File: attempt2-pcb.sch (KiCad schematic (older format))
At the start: 15 parts, among them J1 Conn_01x04, SW1 SW_Push, U1 ATmega32U4-AU, Y1 16MHz

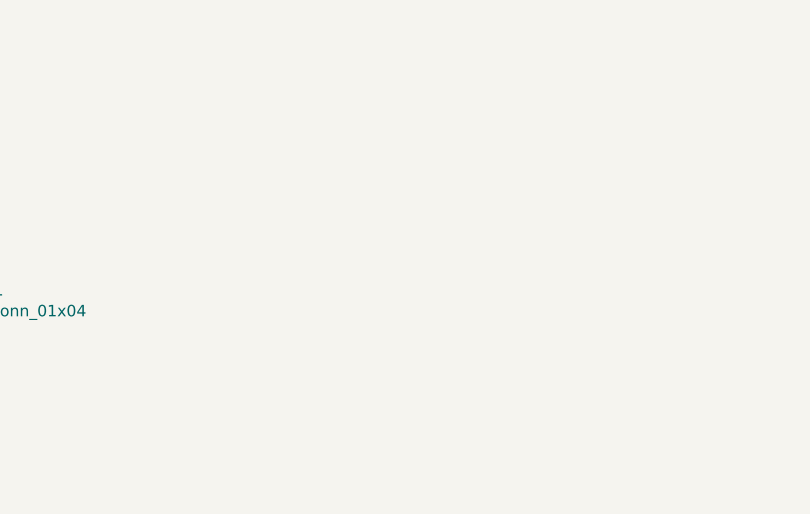
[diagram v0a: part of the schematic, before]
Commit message: PCB prep actually finished
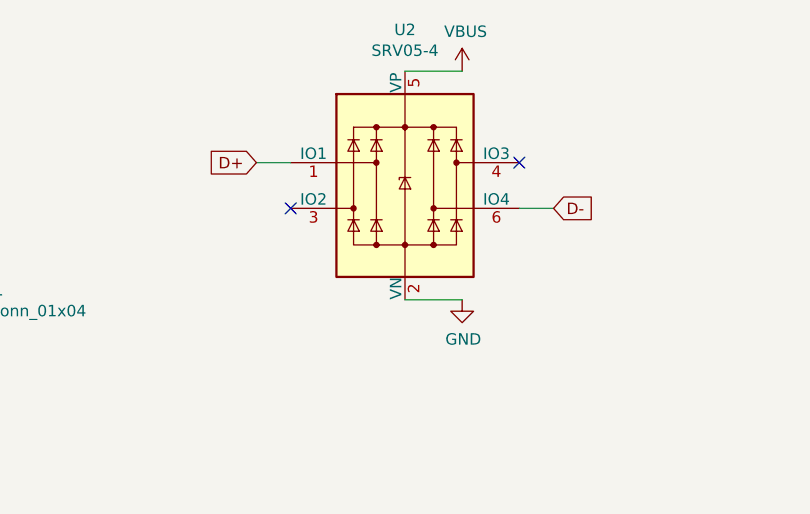
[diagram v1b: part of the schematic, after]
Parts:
- added U2: SRV05-4, Package_TO_SOT_SMD:SOT-23-6, symbol Power_Protection:SRV05-4
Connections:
- net D+: now also U2.1 (IO1)
- net D-: now also U2.6 (IO4)
- net GND: now also U2.2 (VN)
- net VBUS: now also U2.5 (VP)
- no-connect marks 0 -> 2
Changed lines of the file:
@@
 Text GLabel 1050 2350 0    50   Input ~ 0
 D+
+$Comp
+L Power_Protection:SRV05-4 U2
+U 1 1 6234A89E
+P 3300 1800
+F 0 "U2" H 3300 2481 50  0000 C CNN
+F 1 "SRV05-4" H 3300 2390 50  0000 C CNN
+F 2 "Package_TO_SOT_SMD:SOT-23-6" H 4000 1350 50  0001 C CNN
+F 3 "http://www.onsemi.com/pub/Collateral/SRV05-4-D.PDF" H 3300 1800 50  0001 C CNN
+	1    3300 1800
+	1    0    0    -1
+$EndComp
+NoConn ~ 3800 1700
+NoConn ~ 2800 1900
+Wire Wire Line
+	2800 1700 2650 1700
+Wire Wire Line
+	3800 1900 3950 1900
+Text GLabel 2650 1700 0    50   Input ~ 0
+D+
+Text GLabel 3950 1900 2    50   Input ~ 0
+D-
+Wire Wire Line
+	3300 2300 3550 2300
+$Comp
+L power:GND #PWR0113
+U 1 1 623564EB
+P 3550 2300
+F 0 "#PWR0113" H 3550 2050 50  0001 C CNN
+F 1 "GND" H 3555 2127 50  0000 C CNN
+F 2 "" H 3550 2300 50  0001 C CNN
+F 3 "" H 3550 2300 50  0001 C CNN
+	1    3550 2300
+	1    0    0    -1
+$EndComp
+Wire Wire Line
+	3300 1300 3550 1300
+$Comp
+L power:VBUS #PWR0114
+U 1 1 6235878A
+P 3550 1300
+F 0 "#PWR0114" H 3550 1150 50  0001 C CNN
+F 1 "VBUS" H 3565 1473 50  0000 C CNN
+F 2 "" H 3550 1300 50  0001 C CNN
+F 3 "" H 3550 1300 50  0001 C CNN
+	1    3550 1300
+	1    0    0    -1
+$EndComp
 $EndSCHEMATC

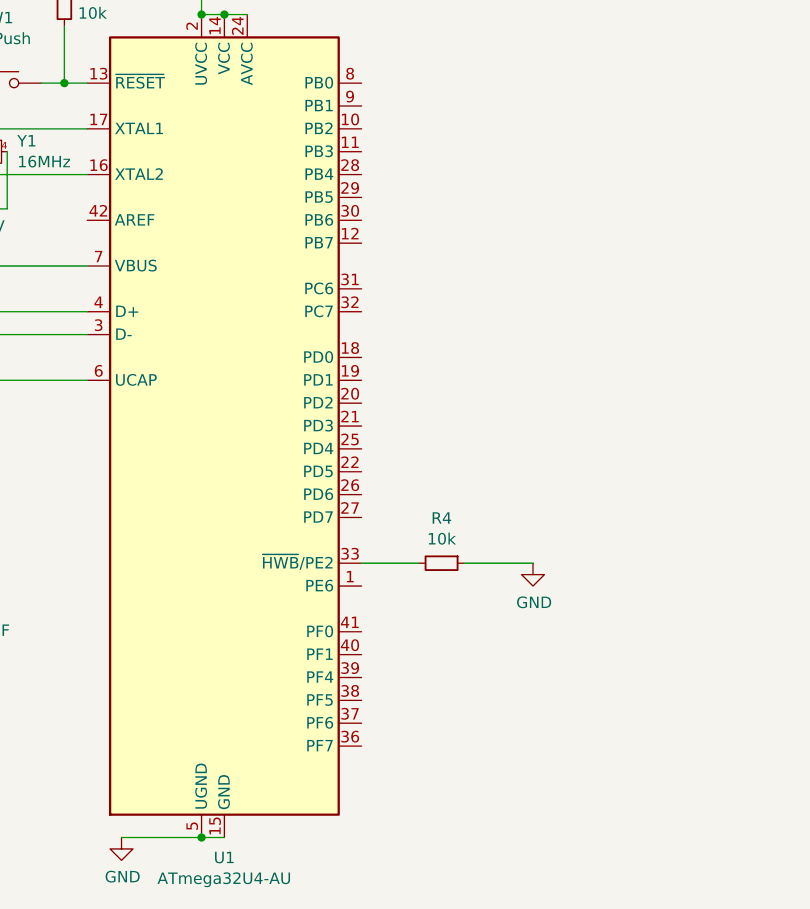
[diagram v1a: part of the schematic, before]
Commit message: Rough Draft Finished
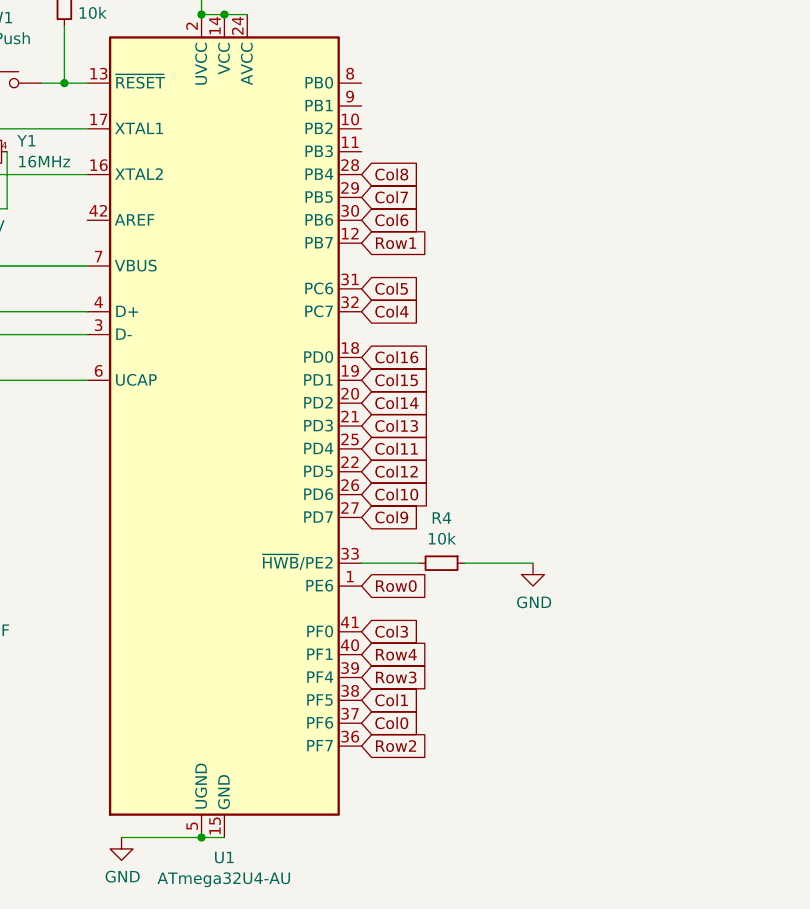
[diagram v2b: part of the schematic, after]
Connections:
- net Row0: now reaches U1.1 (PE6)
- net Row1: now reaches U1.12 (PB7)
- net Col16: now reaches U1.18 (PD0)
- net Col15: now reaches U1.19 (PD1)
- net Col14: now reaches U1.20 (PD2)
- net Col13: now reaches U1.21 (PD3)
- net Col12: now reaches U1.22 (PD5)
- net Col11: now reaches U1.25 (PD4)
- net Col10: now reaches U1.26 (PD6)
- net Col9: now reaches U1.27 (PD7)
- net Col8: now reaches U1.28 (PB4)
- net Col7: now reaches U1.29 (PB5)
- net Col6: now reaches U1.30 (PB6)
- net Col5: now reaches U1.31 (PC6)
- net Col4: now reaches U1.32 (PC7)
- net Row2: now reaches U1.36 (PF7)
- net Col0: now reaches U1.37 (PF6)
- net Col1: now reaches U1.38 (PF5)
- net Row3: now reaches U1.39 (PF4)
- net Row4: now reaches U1.40 (PF1)
- net Col3: now reaches U1.41 (PF0)
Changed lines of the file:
@@
 	0    1    1    0
+$EndComp
+$Comp
+L power:GND #PWR0102
+U 1 1 6228E976
+P 2400 7450
+F 0 "#PWR0102" H 2400 7200 50  0001 C CNN
+F 1 "GND" H 2405 7277 50  0000 C CNN
+F 2 "" H 2400 7450 50  0001 C CNN
+F 3 "" H 2400 7450 50  0001 C CNN
+	1    2400 7450
+	1    0    0    -1
+$EndComp
+Wire Wire Line
+	2750 3700 2750 3850
+$Comp
+L power:+5V #PWR0101
+U 1 1 622836F5
+P 2750 3700
+F 0 "#PWR0101" H 2750 3550 50  0001 C CNN
+F 1 "+5V" H 2765 3873 50  0000 C CNN
+F 2 "" H 2750 3700 50  0001 C CNN
+F 3 "" H 2750 3700 50  0001 C CNN
+	1    2750 3700
+	1    0    0    -1
+$EndComp
+$Sheet
+S 9500 4950 1600 1450
+U 62363975
+F0 "switch matrix" 50
+F1 "matrix.sch" 50
+$EndSheet
+$Comp
+L Connector_Generic:Conn_01x04 J1
+U 1 1 626DFEAA
+P 1400 2250
+F 0 "J1" H 1480 2242 50  0000 L CNN
+F 1 "Conn_01x04" H 1480 2151 50  0000 L CNN
+F 2 "random-keyboard-parts:JST-SR-4" H 1400 2250 50  0001 C CNN
+F 3 "~" H 1400 2250 50  0001 C CNN
+	1    1400 2250
+	1    0    0    -1
+$EndComp
+Wire Wire Line
+	1200 2150 1050 2150
+Wire Wire Line
+	1050 2150 1050 2050
+$Comp
+L power:VBUS #PWR0111
+U 1 1 626E380F
+P 1050 2050
+F 0 "#PWR0111" H 1050 1900 50  0001 C CNN
+F 1 "VBUS" H 1065 2223 50  0000 C CNN
+F 2 "" H 1050 2050 50  0001 C CNN
+F 3 "" H 1050 2050 50  0001 C CNN
+	1    1050 2050
+	1    0    0    -1
+$EndComp
+Wire Wire Line
+	1200 2450 1050 2450
+Wire Wire Line
+	1050 2450 1050 2550
+$Comp
+L power:GND #PWR0112
+U 1 1 626E5F38
+P 1050 2550
+F 0 "#PWR0112" H 1050 2300 50  0001 C CNN
+F 1 "GND" H 1055 2377 50  0000 C CNN
+F 2 "" H 1050 2550 50  0001 C CNN
+F 3 "" H 1050 2550 50  0001 C CNN
+	1    1050 2550
+	1    0    0    -1
+$EndComp
+Wire Wire Line
+	1200 2350 1050 2350
+Wire Wire Line
+	1200 2250 1050 2250
+Text GLabel 1050 2250 0    50   Input ~ 0
+D-
+Text GLabel 1050 2350 0    50   Input ~ 0
+D+
+$Comp
+L Power_Protection:SRV05-4 U2
+U 1 1 6234A89E
+P 3300 1800
+F 0 "U2" H 3300 2481 50  0000 C CNN
+F 1 "SRV05-4" H 3300 2390 50  0000 C CNN
+F 2 "Package_TO_SOT_SMD:SOT-23-6" H 4000 1350 50  0001 C CNN
+F 3 "http://www.onsemi.com/pub/Collateral/SRV05-4-D.PDF" H 3300 1800 50  0001 C CNN
+	1    3300 1800
+	1    0    0    -1
+$EndComp
+NoConn ~ 3800 1700
+NoConn ~ 2800 1900
+Wire Wire Line
+	2800 1700 2650 1700
+Wire Wire Line
+	3800 1900 3950 1900
+Text GLabel 2650 1700 0    50   Input ~ 0
+D+
+Text GLabel 3950 1900 2    50   Input ~ 0
+D-
+Wire Wire Line
+	3300 2300 3550 2300
+$Comp
+L power:GND #PWR0113
+U 1 1 623564EB
+P 3550 2300
+F 0 "#PWR0113" H 3550 2050 50  0001 C CNN
+F 1 "GND" H 3555 2127 50  0000 C CNN
+F 2 "" H 3550 2300 50  0001 C CNN
+F 3 "" H 3550 2300 50  0001 C CNN
+	1    3550 2300
+	1    0    0    -1
+$EndComp
+Wire Wire Line
+	3300 1300 3550 1300
+$Comp
+L power:VBUS #PWR0114
+U 1 1 6235878A
+P 3550 1300
+F 0 "#PWR0114" H 3550 1150 50  0001 C CNN
+F 1 "VBUS" H 3565 1473 50  0000 C CNN
+F 2 "" H 3550 1300 50  0001 C CNN
+F 3 "" H 3550 1300 50  0001 C CNN
+	1    3550 1300
+	1    0    0    -1
+$EndComp
+Text GLabel 3450 5450 2    50   Input ~ 0
+Col15
+Text GLabel 3450 5550 2    50   Input ~ 0
+Col14
+Text GLabel 3450 5650 2    50   Input ~ 0
+Col13
+Text GLabel 3450 5750 2    50   Input ~ 0
+Col11
+Text GLabel 3450 5950 2    50   Input ~ 0
+Col10
+Text GLabel 3450 6050 2    50   Input ~ 0
+Col9
+Text GLabel 3450 5850 2    50   Input ~ 0
+Col12
+Connection ~ 2750 3850
+Wire Wire Line
+	2750 3850 2850 3850
+Wire Wire Line
+	2850 3850 2950 3850
+Connection ~ 2850 3850
+Wire Wire Line
+	2400 7450 2750 7450
+Wire Wire Line
+	2750 7450 2850 7450
+Connection ~ 2750 7450
+$Comp
+L MCU_Microchip_ATmega:ATmega32U4-AU U1
+U 1 1 6227D02D
+P 2850 5650
+F 0 "U1" H 2850 3761 50  0000 C CNN
+F 1 "ATmega32U4-AU" H 2850 3670 50  0000 C CNN
+F 2 "Package_QFP:TQFP-44_10x10mm_P0.8mm" H 2850 5650 50  0001 C CIN
+F 3 "http://ww1.microchip.com/downloads/en/DeviceDoc/Atmel-7766-8-bit-AVR-ATmega16U4-32U4_Datasheet.pdf" H 2850 5650 50  0001 C CNN
+	1    2850 5650
+	1    0    0    -1
 $EndComp
 Wire Wire Line
@@
 	0    1    1    0
 $EndComp
-Connection ~ 2750 7450
-Wire Wire Line
-	2750 7450 2850 7450
-Wire Wire Line
-	2400 7450 2750 7450
-$Comp
-L power:GND #PWR0102
-U 1 1 6228E976
-P 2400 7450
-F 0 "#PWR0102" H 2400 7200 50  0001 C CNN
-F 1 "GND" H 2405 7277 50  0000 C CNN
-F 2 "" H 2400 7450 50  0001 C CNN
-F 3 "" H 2400 7450 50  0001 C CNN
-	1    2400 7450
-	1    0    0    -1
-$EndComp
-Connection ~ 2850 3850
-Wire Wire Line
-	2850 3850 2950 3850
-Connection ~ 2750 3850
-Wire Wire Line
-	2750 3850 2850 3850
-Wire Wire Line
-	2750 3700 2750 3850
-$Comp
-L power:+5V #PWR0101
-U 1 1 622836F5
-P 2750 3700
-F 0 "#PWR0101" H 2750 3550 50  0001 C CNN
-F 1 "+5V" H 2765 3873 50  0000 C CNN
-F 2 "" H 2750 3700 50  0001 C CNN
-F 3 "" H 2750 3700 50  0001 C CNN
-	1    2750 3700
-	1    0    0    -1
-$EndComp
-$Comp
-L MCU_Microchip_ATmega:ATmega32U4-AU U1
-U 1 1 6227D02D
-P 2850 5650
-F 0 "U1" H 2850 3761 50  0000 C CNN
-F 1 "ATmega32U4-AU" H 2850 3670 50  0000 C CNN
-F 2 "Package_QFP:TQFP-44_10x10mm_P0.8mm" H 2850 5650 50  0001 C CIN
-F 3 "http://ww1.microchip.com/downloads/en/DeviceDoc/Atmel-7766-8-bit-AVR-ATmega16U4-32U4_Datasheet.pdf" H 2850 5650 50  0001 C CNN
-	1    2850 5650
-	1    0    0    -1
-$EndComp
-$Sheet
-S 9500 4950 1600 1450
-U 62363975
-F0 "switch matrix" 50
-F1 "matrix.sch" 50
-$EndSheet
-$Comp
-L Connector_Generic:Conn_01x04 J1
-U 1 1 626DFEAA
-P 1400 2250
-F 0 "J1" H 1480 2242 50  0000 L CNN
-F 1 "Conn_01x04" H 1480 2151 50  0000 L CNN
-F 2 "random-keyboard-parts:JST-SR-4" H 1400 2250 50  0001 C CNN
-F 3 "~" H 1400 2250 50  0001 C CNN
-	1    1400 2250
-	1    0    0    -1
-$EndComp
-Wire Wire Line
-	1200 2150 1050 2150
-Wire Wire Line
-	1050 2150 1050 2050
-$Comp
-L power:VBUS #PWR0111
-U 1 1 626E380F
-P 1050 2050
-F 0 "#PWR0111" H 1050 1900 50  0001 C CNN
-F 1 "VBUS" H 1065 2223 50  0000 C CNN
-F 2 "" H 1050 2050 50  0001 C CNN
-F 3 "" H 1050 2050 50  0001 C CNN
-	1    1050 2050
-	1    0    0    -1
-$EndComp
-Wire Wire Line
-	1200 2450 1050 2450
-Wire Wire Line
-	1050 2450 1050 2550
-$Comp
-L power:GND #PWR0112
-U 1 1 626E5F38
-P 1050 2550
-F 0 "#PWR0112" H 1050 2300 50  0001 C CNN
-F 1 "GND" H 1055 2377 50  0000 C CNN
-F 2 "" H 1050 2550 50  0001 C CNN
-F 3 "" H 1050 2550 50  0001 C CNN
-	1    1050 2550
-	1    0    0    -1
-$EndComp
-Wire Wire Line
-	1200 2350 1050 2350
-Wire Wire Line
-	1200 2250 1050 2250
-Text GLabel 1050 2250 0    50   Input ~ 0
-D-
-Text GLabel 1050 2350 0    50   Input ~ 0
-D+
-$Comp
-L Power_Protection:SRV05-4 U2
-U 1 1 6234A89E
-P 3300 1800
-F 0 "U2" H 3300 2481 50  0000 C CNN
-F 1 "SRV05-4" H 3300 2390 50  0000 C CNN
-F 2 "Package_TO_SOT_SMD:SOT-23-6" H 4000 1350 50  0001 C CNN
-F 3 "http://www.onsemi.com/pub/Collateral/SRV05-4-D.PDF" H 3300 1800 50  0001 C CNN
-	1    3300 1800
-	1    0    0    -1
-$EndComp
-NoConn ~ 3800 1700
-NoConn ~ 2800 1900
-Wire Wire Line
-	2800 1700 2650 1700
-Wire Wire Line
-	3800 1900 3950 1900
-Text GLabel 2650 1700 0    50   Input ~ 0
-D+
-Text GLabel 3950 1900 2    50   Input ~ 0
-D-
-Wire Wire Line
-	3300 2300 3550 2300
-$Comp
-L power:GND #PWR0113
-U 1 1 623564EB
-P 3550 2300
-F 0 "#PWR0113" H 3550 2050 50  0001 C CNN
-F 1 "GND" H 3555 2127 50  0000 C CNN
-F 2 "" H 3550 2300 50  0001 C CNN
-F 3 "" H 3550 2300 50  0001 C CNN
-	1    3550 2300
-	1    0    0    -1
-$EndComp
-Wire Wire Line
-	3300 1300 3550 1300
-$Comp
-L power:VBUS #PWR0114
-U 1 1 6235878A
-P 3550 1300
-F 0 "#PWR0114" H 3550 1150 50  0001 C CNN
-F 1 "VBUS" H 3565 1473 50  0000 C CNN
-F 2 "" H 3550 1300 50  0001 C CNN
-F 3 "" H 3550 1300 50  0001 C CNN
-	1    3550 1300
-	1    0    0    -1
-$EndComp
+Text GLabel 3450 6350 2    50   Input ~ 0
+Row0
+Text GLabel 3450 4550 2    50   Input ~ 0
+Col8
+Text GLabel 3450 5350 2    50   Input ~ 0
+Col16
+Text GLabel 3450 4650 2    50   Input ~ 0
+Col7
+Text GLabel 3450 4750 2    50   Input ~ 0
+Col6
+Text GLabel 3450 5050 2    50   Input ~ 0
+Col5
+Text GLabel 3450 5150 2    50   Input ~ 0
+Col4
+Text GLabel 3450 7050 2    50   Input ~ 0
+Row2
+Text GLabel 3450 6550 2    50   Input ~ 0
+Col3
+Text GLabel 3450 4850 2    50   Input ~ 0
+Row1
+Text GLabel 3450 6950 2    50   Input ~ 0
+Col0
+Text GLabel 3450 6850 2    50   Input ~ 0
+Col1
+Text GLabel 3450 6750 2    50   Input ~ 0
+Row3
+Text GLabel 3450 6650 2    50   Input ~ 0
+Row4
 $EndSCHEMATC
